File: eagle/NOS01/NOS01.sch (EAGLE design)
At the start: 41 parts, among them IC1 TL072P, IC2 TL072P, T1 2SC1815, T2 2SC1815

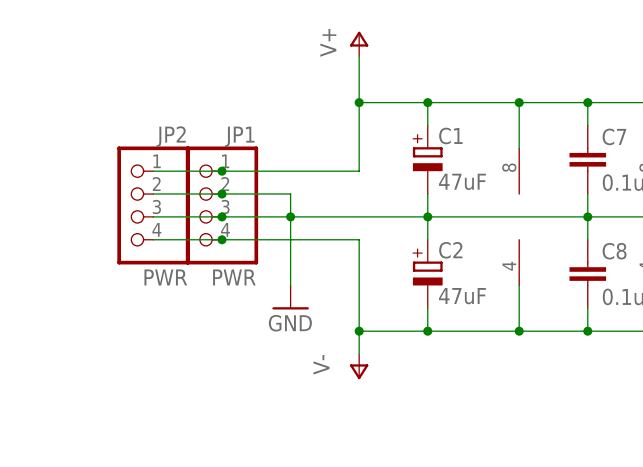
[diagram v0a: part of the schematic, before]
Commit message: Update eagle files
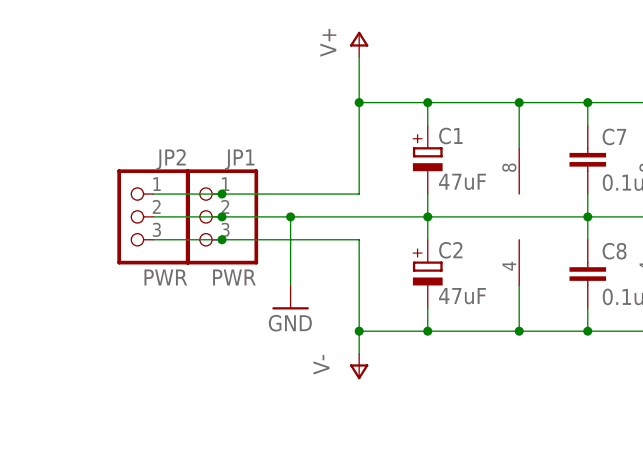
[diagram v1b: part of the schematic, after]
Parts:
- JP1, JP2: device pinhead:PINHD-1X4 -> pinhead:PINHD-1X3
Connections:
- net GND: no longer JP1.3, JP2.3
- net V-: now also JP1.3, JP2.3; no longer JP1.4, JP2.4
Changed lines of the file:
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@@
 </classes>
 <parts>
-<part name="JP1" library="pinhead" deviceset="PINHD-1X4" device="" value="PWR"/>
-<part name="JP2" library="pinhead" deviceset="PINHD-1X4" device="" value="PWR"/>
 <part name="P+1" library="supply1" deviceset="V+" device=""/>
 <part name="P-1" library="supply1" deviceset="V-" device=""/>
@@
 <part name="JP9" library="pinhead" deviceset="PINHD-1X2" device="" value="BLUE"/>
 <part name="FRAME1" library="frames" deviceset="A4L-LOC" device=""/>
+<part name="JP1" library="pinhead" deviceset="PINHD-1X3" device="" value="PWR"/>
+<part name="JP2" library="pinhead" deviceset="PINHD-1X3" device="" value="PWR"/>
 </parts>
 <sheets>
@@
 </plain>
 <instances>
-<instance part="JP1" gate="A" x="40.64" y="139.7" rot="MR0"/>
-<instance part="JP2" gate="A" x="33.02" y="139.7" rot="MR0"/>
 <instance part="P+1" gate="1" x="58.42" y="160.02"/>
 <instance part="P-1" gate="1" x="58.42" y="121.92"/>
@@
 <instance part="JP9" gate="G$1" x="223.52" y="50.8"/>
 <instance part="FRAME1" gate="G$1" x="0" y="0"/>
+<instance part="JP1" gate="A" x="40.64" y="139.7" rot="MR0"/>
+<instance part="JP2" gate="A" x="33.02" y="139.7" rot="MR0"/>
 </instances>
 <busses>
@@
 <net name="GND" class="0">
 <segment>
-<pinref part="JP1" gate="A" pin="2"/>
 <pinref part="GND1" gate="1" pin="GND"/>
-<wire x1="43.18" y1="142.24" x2="50.8" y2="142.24" width="0.1524" layer="91"/>
-<wire x1="50.8" y1="142.24" x2="50.8" y2="139.7" width="0.1524" layer="91"/>
-<pinref part="JP1" gate="A" pin="3"/>
 <wire x1="50.8" y1="139.7" x2="50.8" y2="132.08" width="0.1524" layer="91"/>
-<wire x1="43.18" y1="139.7" x2="50.8" y2="139.7" width="0.1524" layer="91"/>
 <junction x="50.8" y="139.7"/>
 <wire x1="50.8" y1="139.7" x2="66.04" y2="139.7" width="0.1524" layer="91"/>
@@
 <wire x1="66.04" y1="139.7" x2="66.04" y2="137.16" width="0.1524" layer="91"/>
 <junction x="66.04" y="139.7"/>
-<pinref part="JP2" gate="A" pin="2"/>
-<wire x1="35.56" y1="142.24" x2="43.18" y2="142.24" width="0.1524" layer="91"/>
-<junction x="43.18" y="142.24"/>
-<pinref part="JP2" gate="A" pin="3"/>
 <wire x1="35.56" y1="139.7" x2="43.18" y2="139.7" width="0.1524" layer="91"/>
-<junction x="43.18" y="139.7"/>
+<wire x1="43.18" y1="139.7" x2="50.8" y2="139.7" width="0.1524" layer="91"/>
 <wire x1="66.04" y1="139.7" x2="83.82" y2="139.7" width="0.1524" layer="91"/>
 <pinref part="C9" gate="G$1" pin="2"/>
@@
 <pinref part="C7" gate="G$1" pin="2"/>
 <wire x1="83.82" y1="142.24" x2="83.82" y2="139.7" width="0.1524" layer="91"/>
+<pinref part="JP1" gate="A" pin="2"/>
+<junction x="43.18" y="139.7"/>
+<pinref part="JP2" gate="A" pin="2"/>
 </segment>
 <segment>
@@
 <net name="V+" class="0">
 <segment>
-<pinref part="JP1" gate="A" pin="1"/>
-<wire x1="43.18" y1="144.78" x2="58.42" y2="144.78" width="0.1524" layer="91"/>
+<wire x1="35.56" y1="142.24" x2="43.18" y2="142.24" width="0.1524" layer="91"/>
 <pinref part="P+1" gate="1" pin="V+"/>
-<wire x1="58.42" y1="144.78" x2="58.42" y2="152.4" width="0.1524" layer="91"/>
+<wire x1="43.18" y1="142.24" x2="58.42" y2="142.24" width="0.1524" layer="91"/>
+<wire x1="58.42" y1="142.24" x2="58.42" y2="152.4" width="0.1524" layer="91"/>
 <wire x1="58.42" y1="152.4" x2="58.42" y2="157.48" width="0.1524" layer="91"/>
 <wire x1="58.42" y1="152.4" x2="66.04" y2="152.4" width="0.1524" layer="91"/>
@@
 <pinref part="C1" gate="G$1" pin="+"/>
 <wire x1="66.04" y1="152.4" x2="66.04" y2="149.86" width="0.1524" layer="91"/>
-<pinref part="JP2" gate="A" pin="1"/>
-<wire x1="35.56" y1="144.78" x2="43.18" y2="144.78" width="0.1524" layer="91"/>
-<junction x="43.18" y="144.78"/>
 <wire x1="66.04" y1="152.4" x2="76.2" y2="152.4" width="0.1524" layer="91"/>
 <junction x="66.04" y="152.4"/>
@@
 <wire x1="91.44" y1="147.32" x2="91.44" y2="152.4" width="0.1524" layer="91"/>
 <junction x="91.44" y="152.4"/>
+<pinref part="JP1" gate="A" pin="1"/>
+<junction x="43.18" y="142.24"/>
+<pinref part="JP2" gate="A" pin="1"/>
 </segment>
 <segment>
@@
 <net name="V-" class="0">
 <segment>
-<pinref part="JP1" gate="A" pin="4"/>
+<wire x1="35.56" y1="137.16" x2="43.18" y2="137.16" width="0.1524" layer="91"/>
+<pinref part="P-1" gate="1" pin="V-"/>
 <wire x1="43.18" y1="137.16" x2="58.42" y2="137.16" width="0.1524" layer="91"/>
-<pinref part="P-1" gate="1" pin="V-"/>
 <wire x1="58.42" y1="137.16" x2="58.42" y2="127" width="0.1524" layer="91"/>
 <pinref part="C2" gate="G$1" pin="-"/>
@@
 <wire x1="66.04" y1="127" x2="58.42" y2="127" width="0.1524" layer="91"/>
 <junction x="58.42" y="127"/>
-<pinref part="JP2" gate="A" pin="4"/>
-<wire x1="35.56" y1="137.16" x2="43.18" y2="137.16" width="0.1524" layer="91"/>
-<junction x="43.18" y="137.16"/>
 <pinref part="IC1" gate="P" pin="V-"/>
 <wire x1="76.2" y1="132.08" x2="76.2" y2="127" width="0.1524" layer="91"/>
@@
 <wire x1="91.44" y1="132.08" x2="91.44" y2="127" width="0.1524" layer="91"/>
 <junction x="91.44" y="127"/>
-</segment>
-<segment>
+<pinref part="JP1" gate="A" pin="3"/>
+<junction x="43.18" y="137.16"/>
+<pinref part="JP2" gate="A" pin="3"/>
+</segment>
+<segment>
